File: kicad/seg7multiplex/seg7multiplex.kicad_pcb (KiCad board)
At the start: 2 copper layers, 49.5 x 80 mm, 21 parts, among them IC1 ATTINY45-P, J1 USB_A, U1 SN74HC595, U2 SN74HC161, U3 74LS48

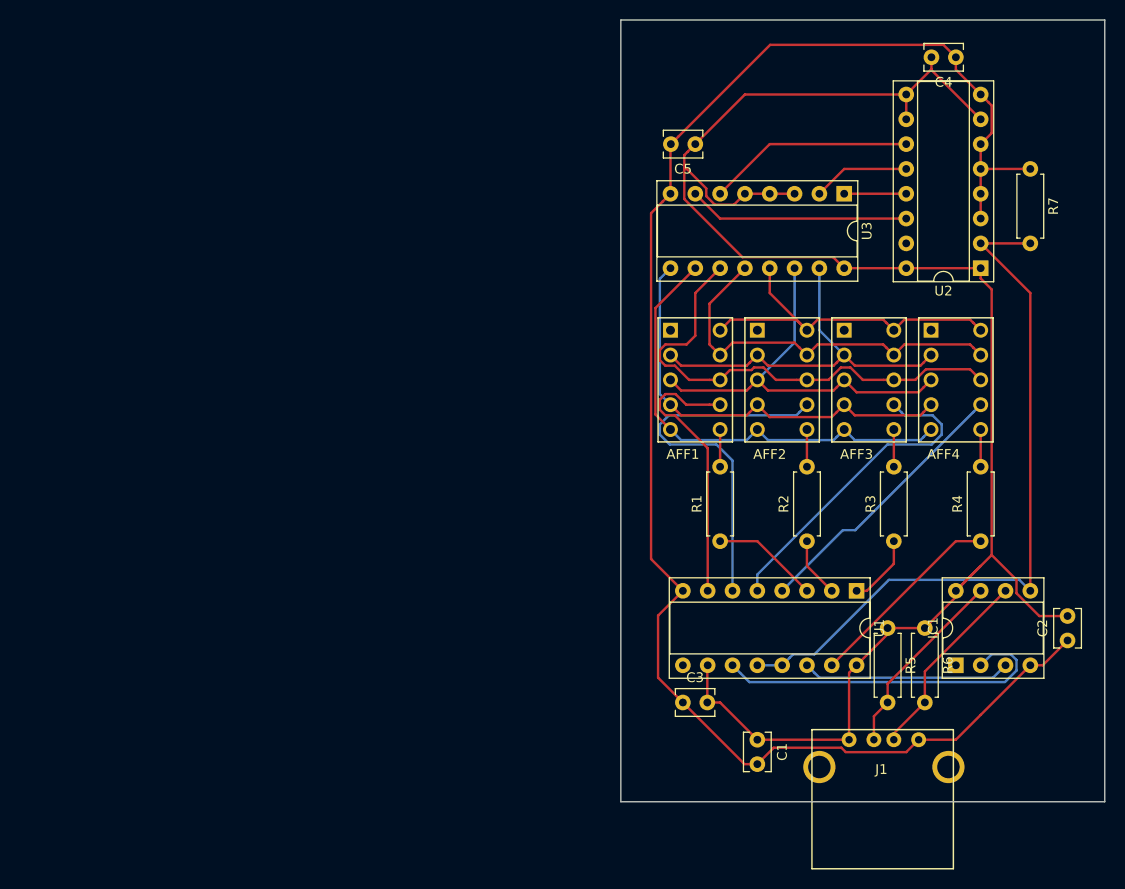
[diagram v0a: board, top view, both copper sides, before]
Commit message: v3!
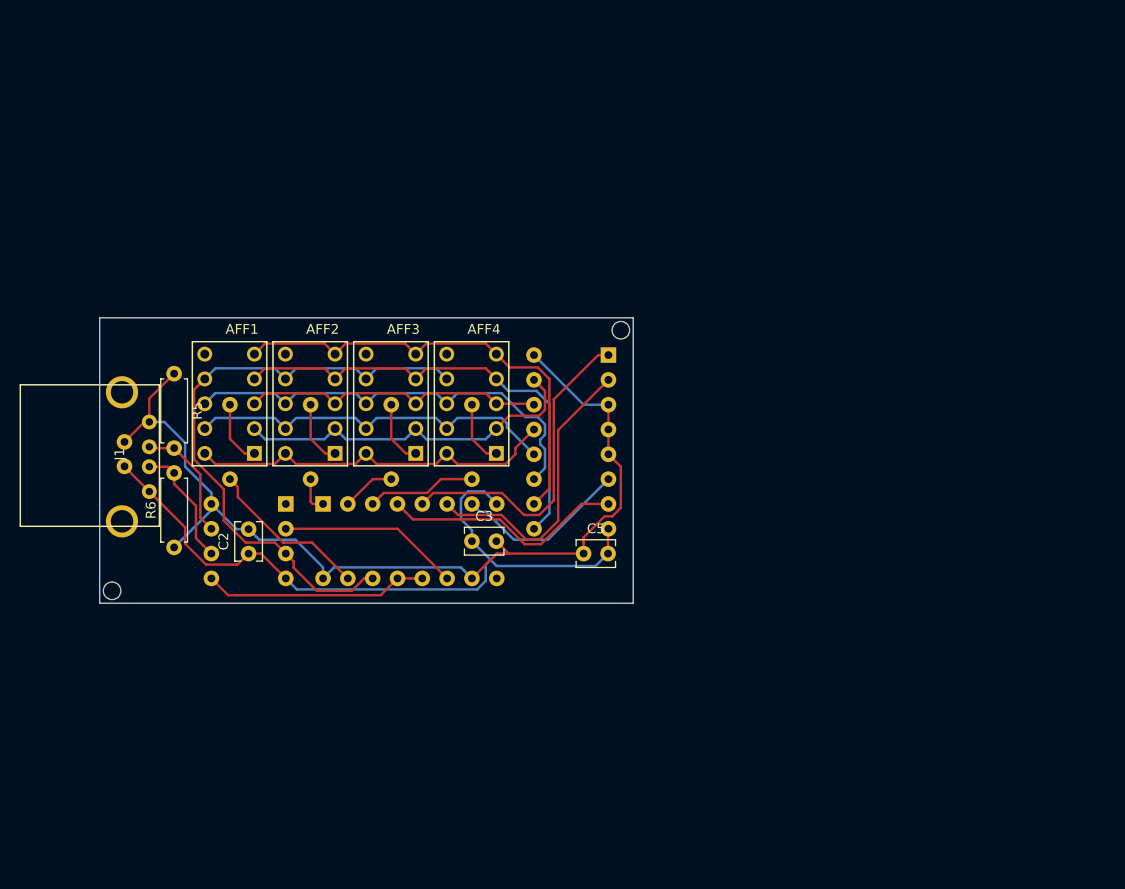
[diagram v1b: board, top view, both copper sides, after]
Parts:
- removed C4: 0.1uF, Capacitor_THT:C_Disc_D3.8mm_W2.6mm_P2.50mm
- removed R7: 10K, Resistor_THT:R_Axial_DIN0207_L6.3mm_D2.5mm_P7.62mm_Horizontal
- removed U2: SN74HC161, Package_DIP:DIP-16_W7.62mm_Socket
- C1, IC1, R1, R2, R3, R4, U1, U3: moved to B.Cu
- moved C2 84.3 mm to (78.7, 100.3)
- moved J1 83.7 mm to (66.0, 90.2), turned to 270 degrees
- moved R5 77.5 mm to (71.1, 81.9)
- moved R6 77.3 mm to (71.1, 99.7), turned to 90 degrees
- moved C1 71.6 mm to (66.0, 88.9)
- moved IC1 70.5 mm to (82.5, 95.2), turned to 180 degrees
- moved U1 55.3 mm to (86.4, 95.2)
- moved R4 52.5 mm to (101.6, 92.7)
- moved R3 51.8 mm to (93.3, 92.7)
- moved R2 51.2 mm to (85.1, 92.7)
- moved R1 50.6 mm to (76.8, 92.7)
- moved AFF4 49.6 mm to (101.6, 85.0), turned to 270 degrees
- moved AFF3 49.0 mm to (93.3, 85.0), turned to 270 degrees
- moved AFF2 48.4 mm to (85.1, 85.0), turned to 270 degrees
- moved AFF1 47.7 mm to (76.8, 85.0), turned to 270 degrees
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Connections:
- net /PB0 renamed /RCLK
- net Net-(IC1-Pad2) renamed /SRCLK
- AFF1 pad 7: /DP3 -> /SER_DP
- AFF2 pad 7: /DP2 -> /SER_DP
- AFF3 pad 7: /DP1 -> /SER_DP
- AFF4 pad 7: /DP0 -> /SER_DP
- IC1 pad 3: Net-(IC1-Pad3) -> /SER_DP
- R1 pad 1: Net-(R1-Pad1) -> /AFF1
- R1 pad 2: Net-(AFF1-Pad6) -> Net-(AFF1-Pad1)
- R2 pad 1: Net-(R2-Pad1) -> /AFF2
- R2 pad 2: Net-(AFF2-Pad6) -> Net-(AFF2-Pad1)
- R3 pad 1: Net-(R3-Pad1) -> /AFF3
- R3 pad 2: Net-(AFF3-Pad6) -> Net-(AFF3-Pad1)
- R4 pad 1: Net-(R4-Pad1) -> /AFF4
- R4 pad 2: Net-(AFF4-Pad6) -> Net-(AFF4-Pad1)
- U1 pad 1: Net-(R3-Pad1) -> /AFF2
- U1 pad 14: Net-(IC1-Pad3) -> /SER_DP
- U1 pad 15: Net-(R4-Pad1) -> /AFF1
- U1 pad 2: Net-(R2-Pad1) -> /AFF3
- U1 pad 3: Net-(R1-Pad1) -> /AFF4
- U1 pad 4: /DP0 -> /DECA
- U1 pad 5: /DP1 -> /DECB
- U1 pad 6: /DP2 -> /DECC
- U1 pad 7: /DP3 -> /DECD
- U3 pad 1: Net-(U2-Pad13) -> /DECB
- U3 pad 2: Net-(U2-Pad12) -> /DECC
- U3 pad 6: Net-(U2-Pad11) -> /DECD
- U3 pad 7: Net-(U2-Pad14) -> /DECA
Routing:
- net GND: track 166.5 -> 74.8 mm
- net VCC: track 183.1 -> 100.6 mm
- net /SER_DP: track 0.00 -> 62.8 mm
- net /RCLK: track 74.8 -> 23.0 mm
- net /DP2: track 38.8 -> 0.00 mm
- net /DECB: track 0.00 -> 33.3 mm
- net /DP1: track 33.2 -> 0.00 mm
- net /DECC: track 0.00 -> 30.2 mm
- net /DP3: track 29.0 -> 0.00 mm
- net /DP0: track 28.2 -> 0.00 mm
- net /DECA: track 0.00 -> 25.0 mm
- net Net-(U2-Pad14): track 22.6 -> 0.00 mm
- net Net-(IC1-Pad3): track 21.4 -> 0.00 mm
- net Net-(U2-Pad11): track 21.2 -> 0.00 mm
- net Net-(R4-Pad1): track 20.5 -> 0.00 mm
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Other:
- board size 49.5 x 80 mm -> 54.6 x 29.2 mm
